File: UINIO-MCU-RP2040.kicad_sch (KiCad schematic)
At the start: 44 parts, among them J1 Conn_01x20_Pin, J2 Conn_01x20_Pin, J3 Conn_01x04_Pin, Q1 DMG1012T, SW1 ~{RESET}, SW2 ~{USB_BOOT}, U1 SGM2019-3.3YN5G, U2 SPI-25-Flash-WSON8, U3 RP2040, Y1 12MHz

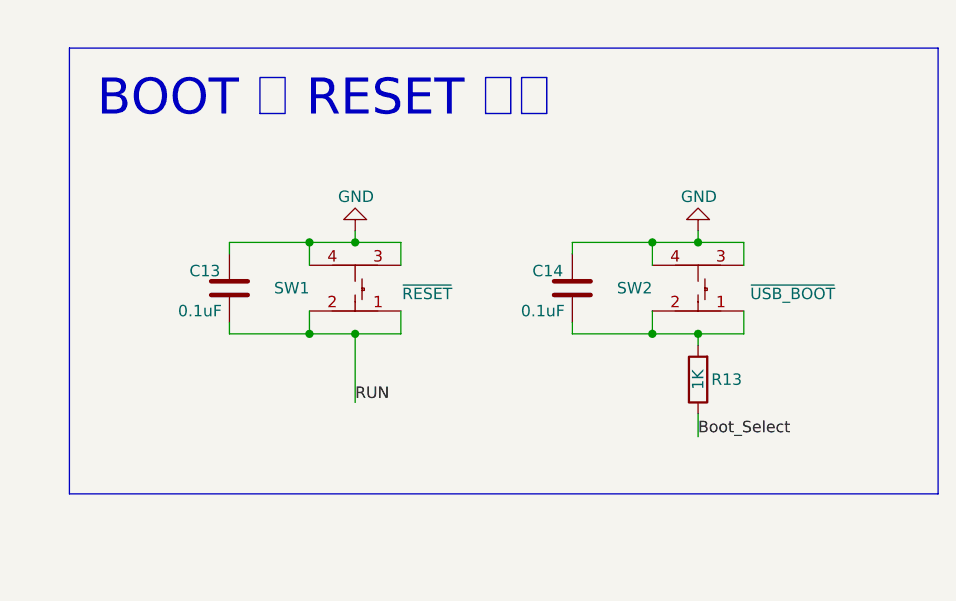
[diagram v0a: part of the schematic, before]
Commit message: Release UINIO-MCU-RP2040 version 2.0.0.
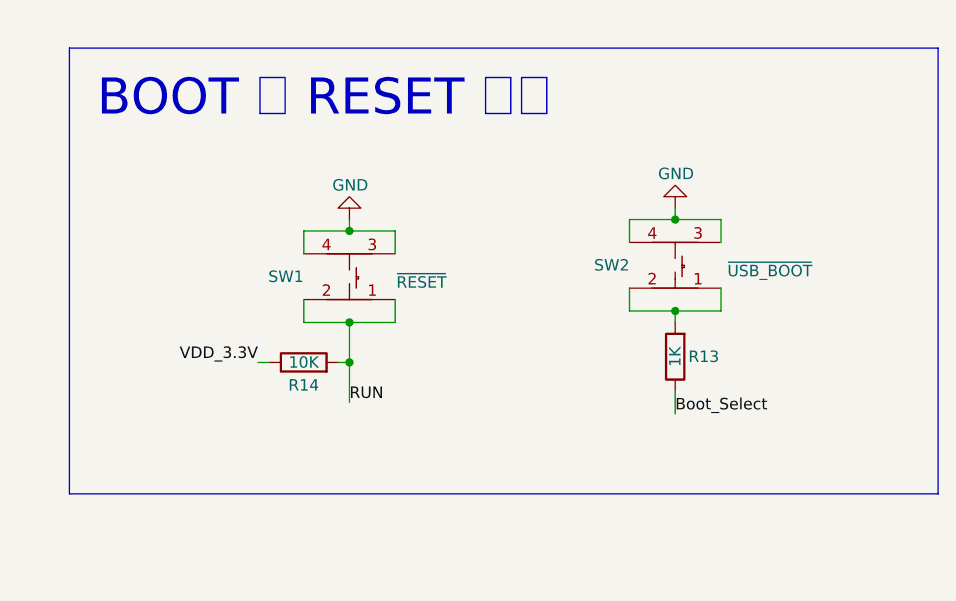
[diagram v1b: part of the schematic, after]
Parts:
- removed C13, C14: 0.1uF, Capacitor_SMD:C_0402_1005Metric, symbol Device:C
- added R14: 10K, Resistor_SMD:R_0402_1005Metric, symbol Device:R
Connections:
- net RUN: now also R14.2
- net VDD_3.3V: now also R14.1
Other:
- moved on the sheet: R13, SW1, SW2

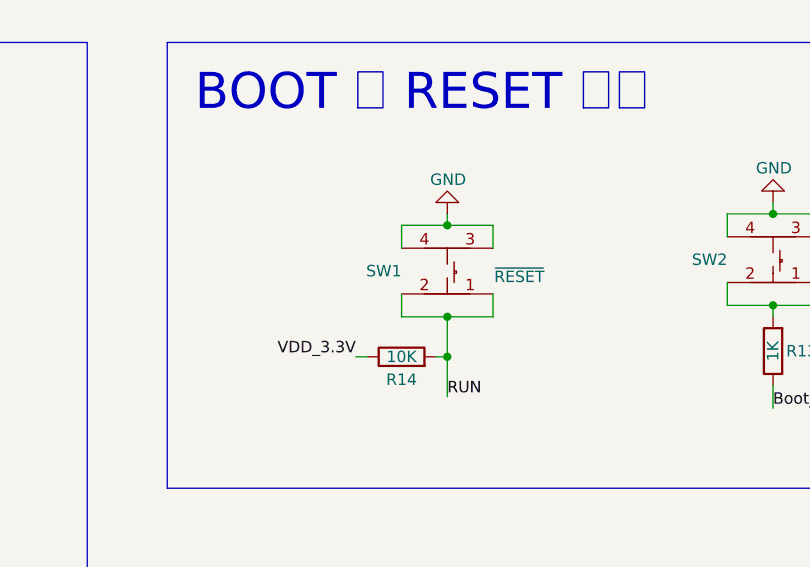
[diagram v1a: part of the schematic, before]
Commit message: Release UINIO-MCU-RP2040 version 2.2.0.
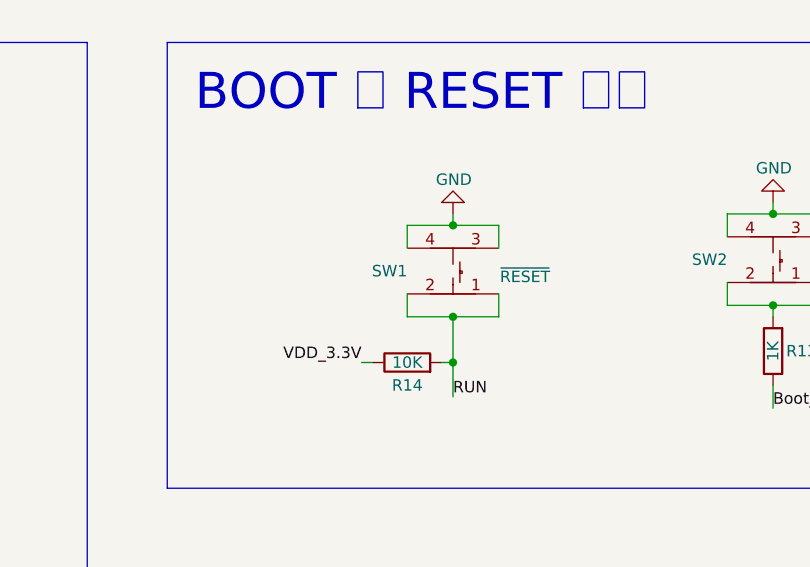
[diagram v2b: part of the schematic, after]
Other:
- moved on the sheet: R14, SW1
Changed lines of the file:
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@@
   (title_block
     (title "UINIO-MCU-RP2040")
-    (date "2024-02-04")
-    (rev "Version 2.0.0")
+    (date "2024-04-13")
+    (rev "Version 2.2.0")
     (company "UinIO.com 电子技术实验室")
   )
@@
   (junction (at 114.3 74.93) (diameter 0) (color 0 0 0 0)
   )
-  (junction (at 332.105 230.505) (diameter 0) (color 0 0 0 0)
+  (junction (at 332.74 231.14) (diameter 0) (color 0 0 0 0)
   )
   (junction (at 248.92 259.08) (diameter 0) (color 0 0 0 0)
@@
   (junction (at 135.89 151.13) (diameter 0) (color 0 0 0 0)
   )
-  (junction (at 332.105 226.06) (diameter 0) (color 0 0 0 0)
+  (junction (at 332.74 226.06) (diameter 0) (color 0 0 0 0)
   )
   (junction (at 118.11 151.13) (diameter 0) (color 0 0 0 0)
@@
   (junction (at 368.3 224.79) (diameter 0) (color 0 0 0 0)
   )
-  (junction (at 332.105 215.9) (diameter 0) (color 0 0 0 0)
+  (junction (at 332.74 215.9) (diameter 0) (color 0 0 0 0)
   )
   (junction (at 63.5 64.77) (diameter 0) (color 0 0 0 0)
@@
     (stroke (width 0) (type default))
   )
-  (wire (pts (xy 332.105 226.06) (xy 332.105 230.505))
+  (wire (pts (xy 332.74 226.06) (xy 332.74 231.14))
     (stroke (width 0) (type default))
   )
@@
     (stroke (width 0) (type default))
   )
-  (wire (pts (xy 332.105 230.505) (xy 332.105 234.95))
+  (wire (pts (xy 332.74 231.14) (xy 332.74 234.95))
     (stroke (width 0) (type default))
   )
@@
     (stroke (width 0) (type default))
   )
-  (wire (pts (xy 337.185 223.52) (xy 337.185 226.06))
+  (wire (pts (xy 337.82 223.52) (xy 337.82 226.06))
     (stroke (width 0) (type default))
   )
@@
     (stroke (width 0) (type default))
   )
-  (wire (pts (xy 332.105 215.9) (xy 337.185 215.9))
+  (wire (pts (xy 332.74 215.9) (xy 337.82 215.9))
     (stroke (width 0) (type default))
   )
@@
     (stroke (width 0) (type default))
   )
-  (wire (pts (xy 332.105 214.63) (xy 332.105 215.9))
+  (wire (pts (xy 332.74 214.63) (xy 332.74 215.9))
     (stroke (width 0) (type default))
   )
@@
     (stroke (width 0) (type default))
   )
-  (wire (pts (xy 337.185 215.9) (xy 337.185 218.44))
+  (wire (pts (xy 337.82 215.9) (xy 337.82 218.44))
     (stroke (width 0) (type default))
   )
@@
     (stroke (width 0) (type default))
   )
-  (wire (pts (xy 330.835 230.505) (xy 332.105 230.505))
+  (wire (pts (xy 331.47 231.14) (xy 332.74 231.14))
     (stroke (width 0) (type default))
   )
@@
     (stroke (width 0) (type default))
   )
-  (wire (pts (xy 327.025 226.06) (xy 332.105 226.06))
-    (stroke (width 0) (type default))
-  )
-  (wire (pts (xy 327.025 218.44) (xy 327.025 215.9))
+  (wire (pts (xy 327.66 226.06) (xy 332.74 226.06))
+    (stroke (width 0) (type default))
+  )
+  (wire (pts (xy 327.66 218.44) (xy 327.66 215.9))
     (stroke (width 0) (type default))
   )
@@
     (stroke (width 0) (type default))
   )
-  (wire (pts (xy 332.105 226.06) (xy 337.185 226.06))
+  (wire (pts (xy 332.74 226.06) (xy 337.82 226.06))
     (stroke (width 0) (type default))
   )
@@
     (stroke (width 0) (type default))
   )
-  (wire (pts (xy 327.025 215.9) (xy 332.105 215.9))
+  (wire (pts (xy 327.66 215.9) (xy 332.74 215.9))
     (stroke (width 0) (type default))
   )
@@
     (stroke (width 0) (type default))
   )
-  (wire (pts (xy 327.025 226.06) (xy 327.025 223.52))
+  (wire (pts (xy 327.66 226.06) (xy 327.66 223.52))
     (stroke (width 0) (type default))
   )
@@
     (stroke (width 0) (type default))
   )
-  (wire (pts (xy 321.945 230.505) (xy 323.215 230.505))
+  (wire (pts (xy 322.58 231.14) (xy 323.85 231.14))
     (stroke (width 0) (type default))
   )
@@
     (effects (font (size 1.27 1.27)) (justify left bottom))
   )
-  (label "VDD_3.3V" (at 321.945 230.505 180) (fields_autoplaced)
+  (label "VDD_3.3V" (at 322.58 231.14 180) (fields_autoplaced)
     (effects (font (size 1.27 1.27)) (justify right bottom))
   )
@@
     (effects (font (size 1.27 1.27)) (justify left bottom))
   )
-  (label "RUN" (at 332.105 234.95 0) (fields_autoplaced)
+  (label "RUN" (at 332.74 234.95 0) (fields_autoplaced)
     (effects (font (size 1.27 1.27)) (justify left bottom))
   )
@@
     )
   )
-  (symbol (lib_id "Device:R") (at 327.025 230.505 90) (unit 1)
-    (in_bom yes) (on_board yes) (dnp no)
-    (property "Reference" "R14" (at 327.025 233.045 90)
+  (symbol (lib_id "Device:R") (at 327.66 231.14 90) (unit 1)
+    (in_bom yes) (on_board yes) (dnp no)
+    (property "Reference" "R14" (at 327.66 233.68 90)
       (effects (font (size 1.27 1.27)))
     )
-    (property "Value" "10K" (at 327.025 230.505 90)
+    (property "Value" "10K" (at 327.66 231.14 90)
       (effects (font (size 1.27 1.27)))
     )
-    (property "Footprint" "Resistor_SMD:R_0402_1005Metric" (at 327.025 232.283 90)
-      (effects (font (size 1.27 1.27)) hide)
-    )
-    (property "Datasheet" "~" (at 327.025 230.505 0)
+    (property "Footprint" "Resistor_SMD:R_0402_1005Metric" (at 327.66 232.918 90)
+      (effects (font (size 1.27 1.27)) hide)
+    )
+    (property "Datasheet" "~" (at 327.66 231.14 0)
       (effects (font (size 1.27 1.27)) hide)
     )
@@
     )
   )
-  (symbol (lib_id "Uinio:Key_YTS_A016S_1") (at 332.105 220.98 180) (unit 1)
-    (in_bom yes) (on_board yes) (dnp no)
-    (property "Reference" "SW1" (at 327.025 220.98 0)
+  (symbol (lib_id "Uinio:Key_YTS_A016S_1") (at 332.74 220.98 180) (unit 1)
+    (in_bom yes) (on_board yes) (dnp no)
+    (property "Reference" "SW1" (at 327.66 220.98 0)
       (effects (font (size 1.27 1.27)) (justify left))
     )
-    (property "Value" "~{RESET}" (at 342.9 221.615 0)
+    (property "Value" "~{RESET}" (at 343.535 221.615 0)
       (effects (font (size 1.27 1.27)) (justify left))
     )
-    (property "Footprint" "Uinio:KEY-SMD_4P-L4.2-W3.4-P2.15-LS4.7" (at 332.105 223.5962 0)
-      (effects (font (size 1.27 1.27)) hide)
-    )
-    (property "Datasheet" "" (at 332.105 218.5162 0)
-      (effects (font (size 1.27 1.27)) hide)
-    )
-    (property "SuppliersPartNumber" "C2910676" (at 332.105 213.4362 0)
-      (effects (font (size 1.27 1.27)) hide)
-    )
-    (property "uuid" "std:78dd57beb35d4dda9340821b45cb0336" (at 332.105 213.4362 0)
+    (property "Footprint" "Uinio:KEY-SMD_4P-L4.2-W3.4-P2.15-LS4.7" (at 332.74 223.5962 0)
+      (effects (font (size 1.27 1.27)) hide)
+    )
+    (property "Datasheet" "" (at 332.74 218.5162 0)
+      (effects (font (size 1.27 1.27)) hide)
+    )
+    (property "SuppliersPartNumber" "C2910676" (at 332.74 213.4362 0)
+      (effects (font (size 1.27 1.27)) hide)
+    )
+    (property "uuid" "std:78dd57beb35d4dda9340821b45cb0336" (at 332.74 213.4362 0)
       (effects (font (size 1.27 1.27)) hide)
     )
@@
     )
   )
-  (symbol (lib_id "power:GND") (at 332.105 214.63 180) (unit 1)
-    (in_bom yes) (on_board yes) (dnp no)
-    (property "Reference" "#PWR027" (at 332.105 208.28 0)
-      (effects (font (size 1.27 1.27)) hide)
-    )
-    (property "Value" "GND" (at 330.2 210.82 0)
+  (symbol (lib_id "power:GND") (at 332.74 214.63 180) (unit 1)
+    (in_bom yes) (on_board yes) (dnp no)
+    (property "Reference" "#PWR027" (at 332.74 208.28 0)
+      (effects (font (size 1.27 1.27)) hide)
+    )
+    (property "Value" "GND" (at 330.835 210.82 0)
       (effects (font (size 1.27 1.27)) (justify right))
     )
-    (property "Footprint" "" (at 332.105 214.63 0)
-      (effects (font (size 1.27 1.27)) hide)
-    )
-    (property "Datasheet" "" (at 332.105 214.63 0)
-      (effects (font (size 1.27 1.27)) hide)
-    )
+    (property "Footprint" "" (at 332.74 214.63 0)
+      (effects (font (size 1.27 1.27)) hide)
+    )
+    (property "Datasheet" "" (at 332.74 214.63 0)
+      (effects (font (size 1.27 1.27)) hide)
+    )
